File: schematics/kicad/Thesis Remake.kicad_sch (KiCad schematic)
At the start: 109 parts, among them J1 SJ2-35853B-SMT-TR, J2 Conn_01x18, J3 Conn_01x18, J4 Conn_01x01_Pin, J5 Conn_01x01_Pin, J6 Conn_01x01_Pin, J7 Conn_01x01_Pin, Q1 MMBT7002K, U10 MCP6001-OT, U11 MCP6001-OT, U2 PCM5102, U3 SN74LVC1G3157, U4 LM78M05_TO220, U5 RT9080-33GJ5, U6 LM2940CT-5.0_MOD, U7 TPA711, U8 LM2940CT-5.0_MOD, U9 MCP6001-OT

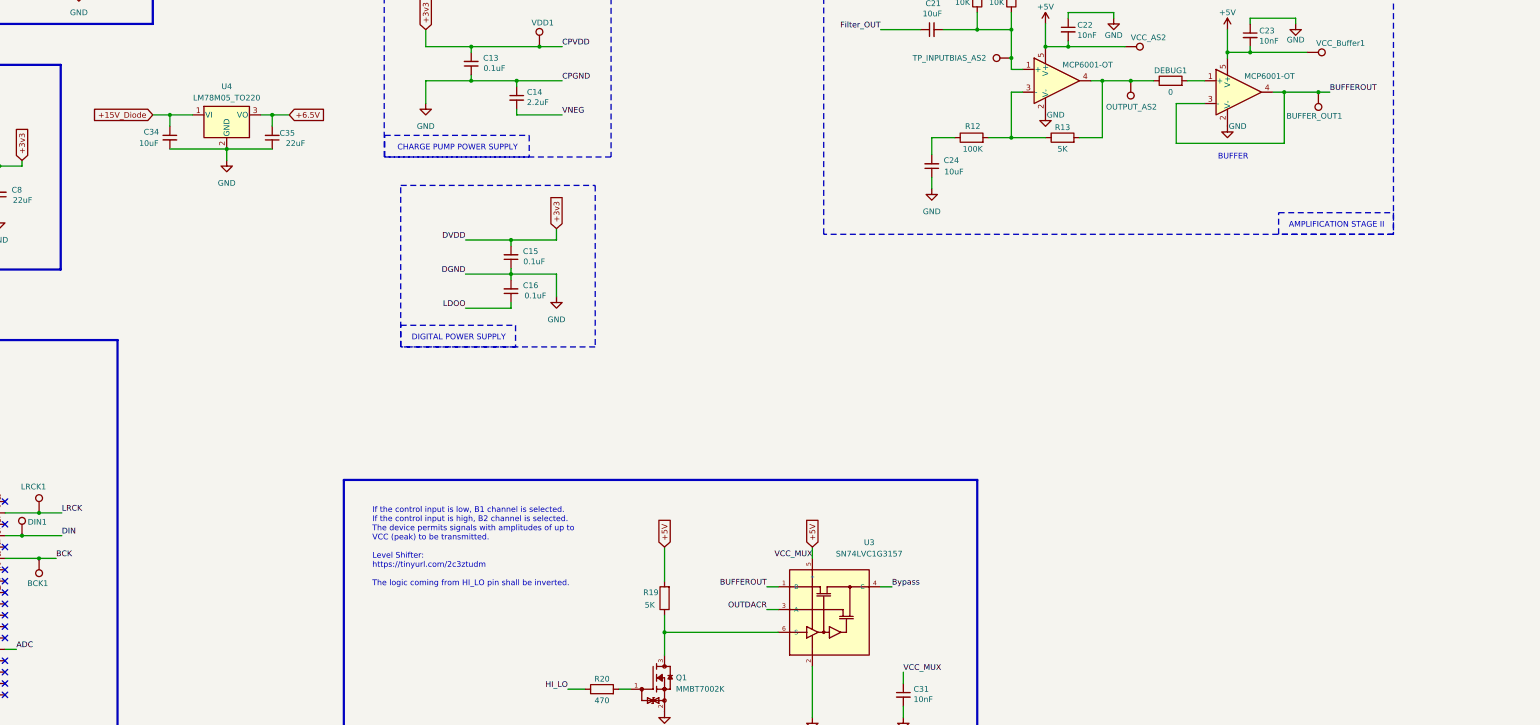
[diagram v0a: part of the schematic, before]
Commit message: Updated schematic in main
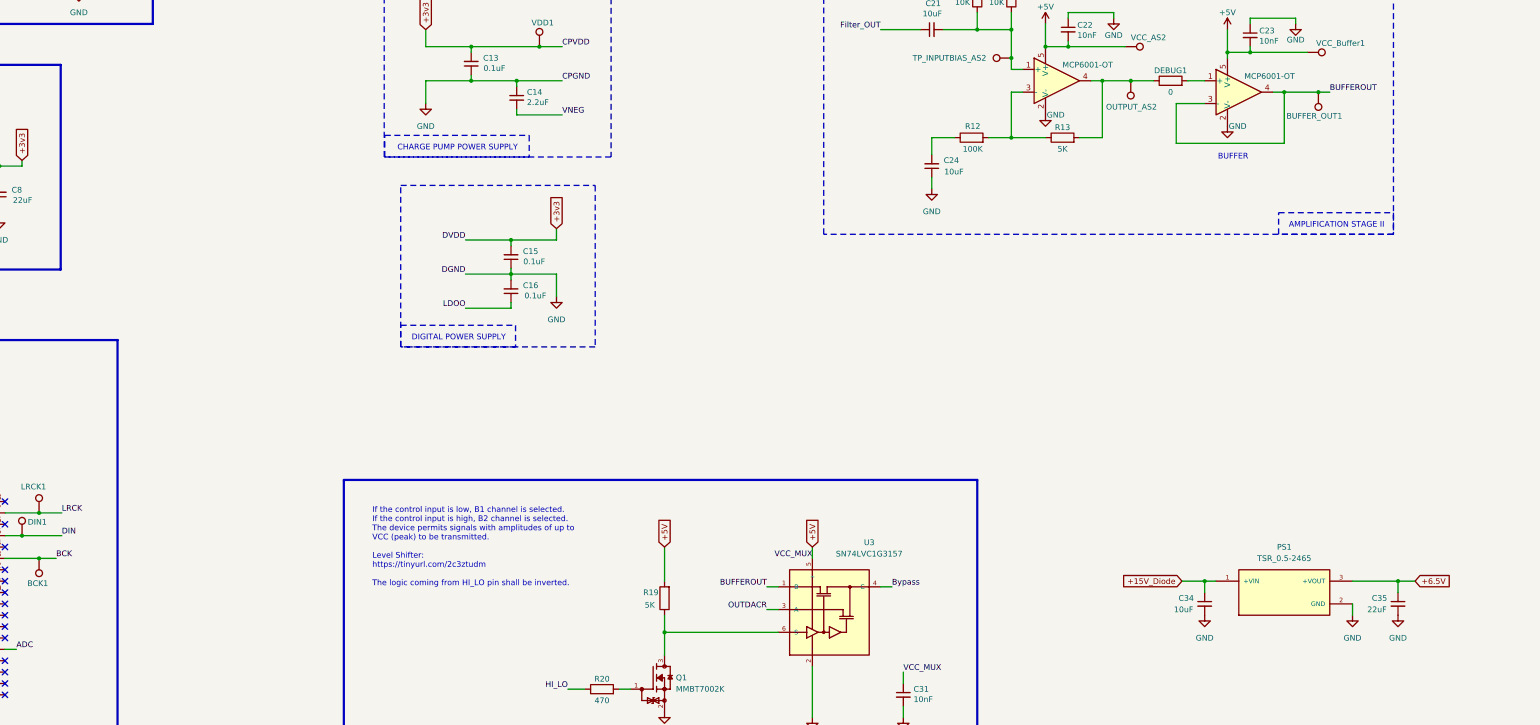
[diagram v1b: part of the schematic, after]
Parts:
- removed U4: LM78M05_TO220, Package_TO_SOT_THT:TO-220-3_Vertical, symbol Regulator_Linear:LM78M05_TO220
- added PS1: TSR_0.5-2465, TSR_0.5-2465:CONV_TSR_0.5-2465, symbol TSR_0.5-2465:TSR_0.5-2465
- C35: Comments 6.3 VDC, 22uF, 1206, X7R -> 16V, X7R, 1206; Description_1 regulation during transients, datasheet recommendation -> input/gnd; OC_Mouser 963-LMK316ABJ226MLHT -> 581-1206YC106KAT4A
- Vo-1: footprint TestPoint:TestPoint_Pad_1.5x1.5mm -> TestPoint:TestPoint_Pad_2.5x2.5mm
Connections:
- net +15V_Diode: now also PS1.1 (+VIN)
- net +6.5V: now also C35.1, PS1.3 (+VOUT); no longer C35.2
- net GND: now also C35.2, PS1.2 (GND); no longer C35.1
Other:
- moved on the sheet: C34
